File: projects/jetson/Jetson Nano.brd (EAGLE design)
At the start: 120 x 100 mm, 20 parts

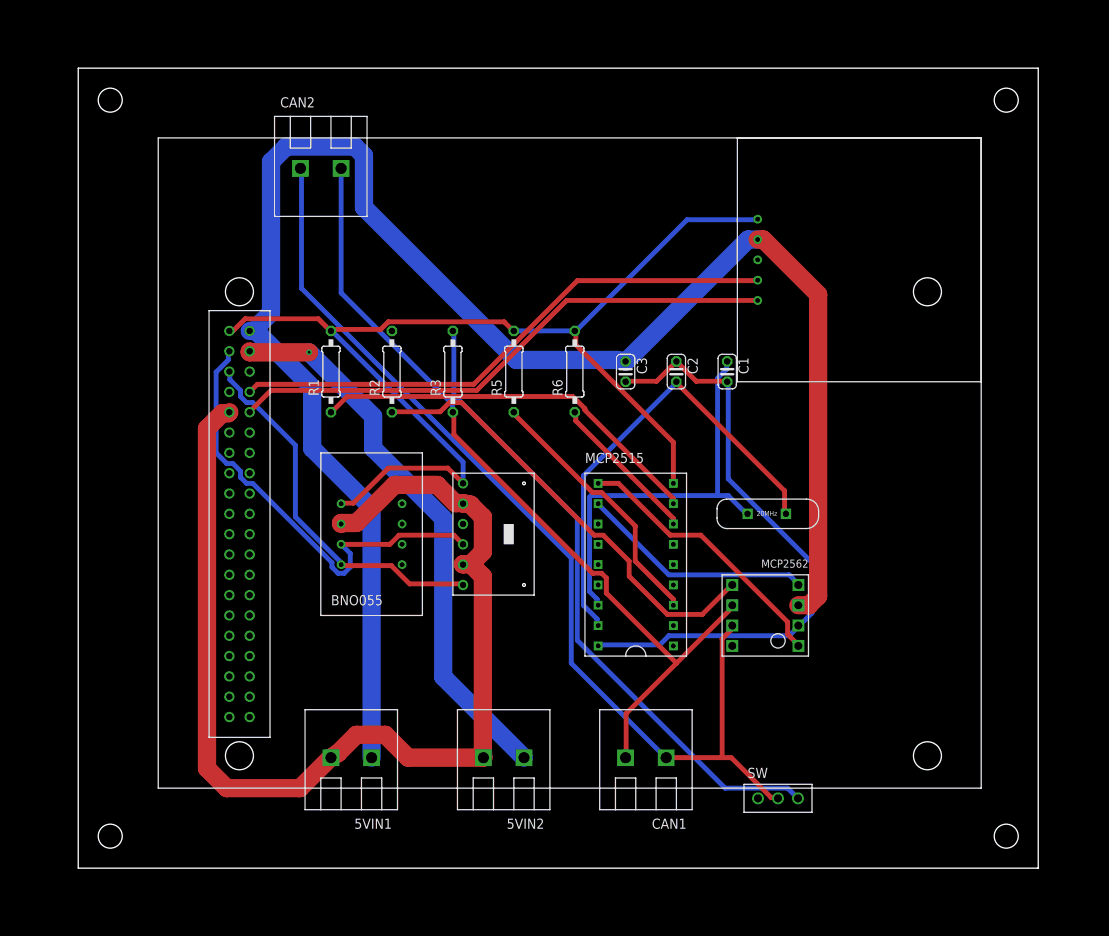
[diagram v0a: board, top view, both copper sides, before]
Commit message: wakuwaku
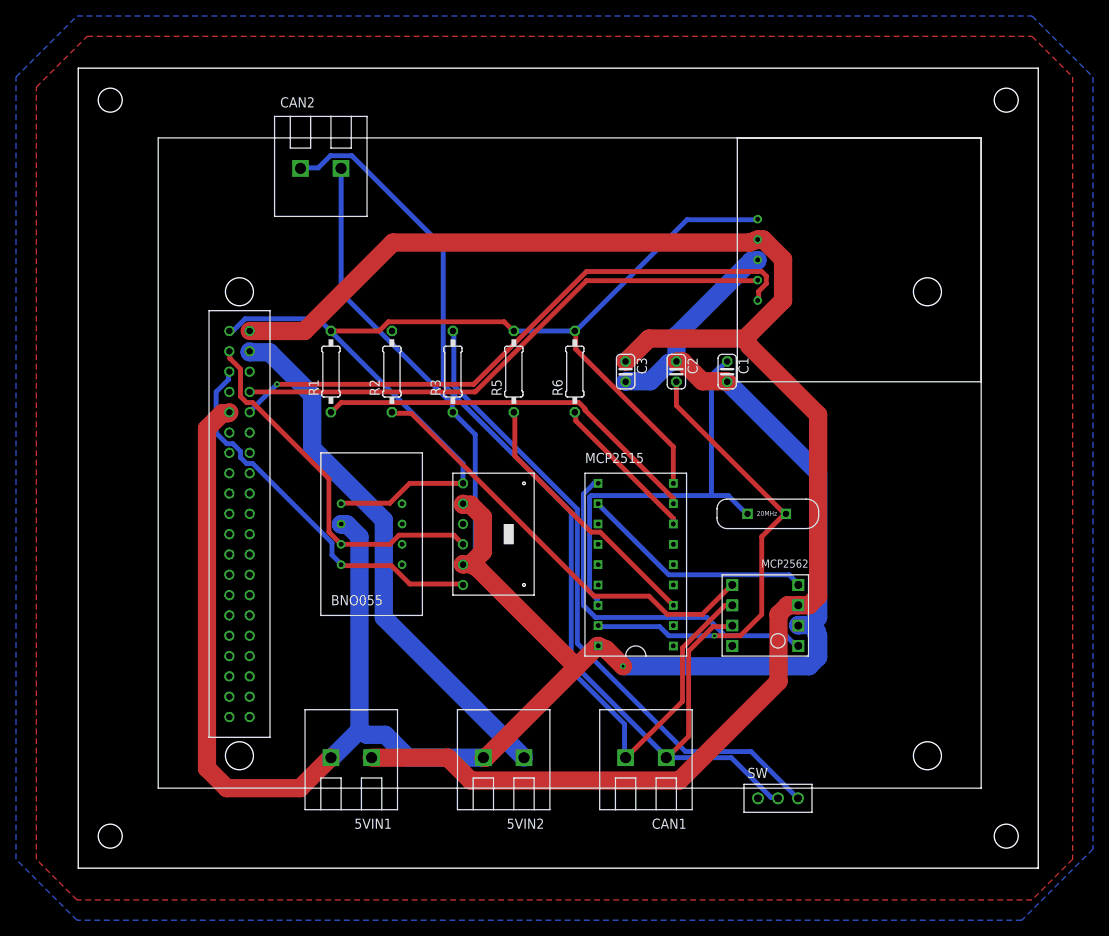
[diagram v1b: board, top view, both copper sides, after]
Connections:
- removed net GND_1: 5VIN1.P$2, 5VIN2.P$2, JN1.GND-2, U$1.GND, U$1.SDO, U$2.2_GND
- removed net V-: C1.2, C2.1, C3.2, MCP1.VSS, U$4.VSS
- new net GND: 5VIN1.P$2, 5VIN2.P$2, C1.2, C2.1, C3.2, JN1.GND-2, MCP1.VSS, U$1.GND, U$1.SDO, U$2.2_GND, U$3.GND, U$4.VSS
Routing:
- net GND: track 0.00 -> 265.1 mm, vias 0 -> 1
- net GND_1: track 139.4 -> 0.00 mm
- net V-: track 76.6 -> 0.00 mm
- net N$8: track 34.4 -> 45.3 mm
- net N$3: track 57.0 -> 46.5 mm
- net CAN_H2: track 125.7 -> 136.0 mm
- net N$16: track 104.6 -> 113.6 mm
- net +5V_1: track 215.8 -> 207.7 mm
- net N$12: track 69.3 -> 75.7 mm, vias 0 -> 1
- net 5V_2: track 69.4 -> 66.5 mm, vias 1 -> 0
- net N$14: track 56.6 -> 54.5 mm
- net N$4: track 46.8 -> 48.6 mm
- net +3V3: track 142.2 -> 140.5 mm
- net N$13: track 49.6 -> 49.0 mm
- net N$7: track 58.4 -> 58.3 mm, vias 0 -> 1
- added copper zone on layer 1, net GND
- added copper zone on layer 16, net GND
